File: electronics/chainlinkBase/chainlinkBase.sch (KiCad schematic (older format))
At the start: 50 parts, among them J101 Power In, J102 RELAY, J103 Power In, J104 RS485, J105 RS485, J106 Logic Power Out, J107 UART, J108 Output, J109 Output, J110 Output, J111 Conn_01x06_Male, J112 Conn_01x06_Male, SW101 SW_DIP_x04, U101 AP7361C-33E, U102 TPL7407L, U103 Buck, U104 TTGO_TDisplay, U105 MCP23017_SS, U106 SN74LV1T34DBV, U107 SP485, U108 SN74LV1T34DBV

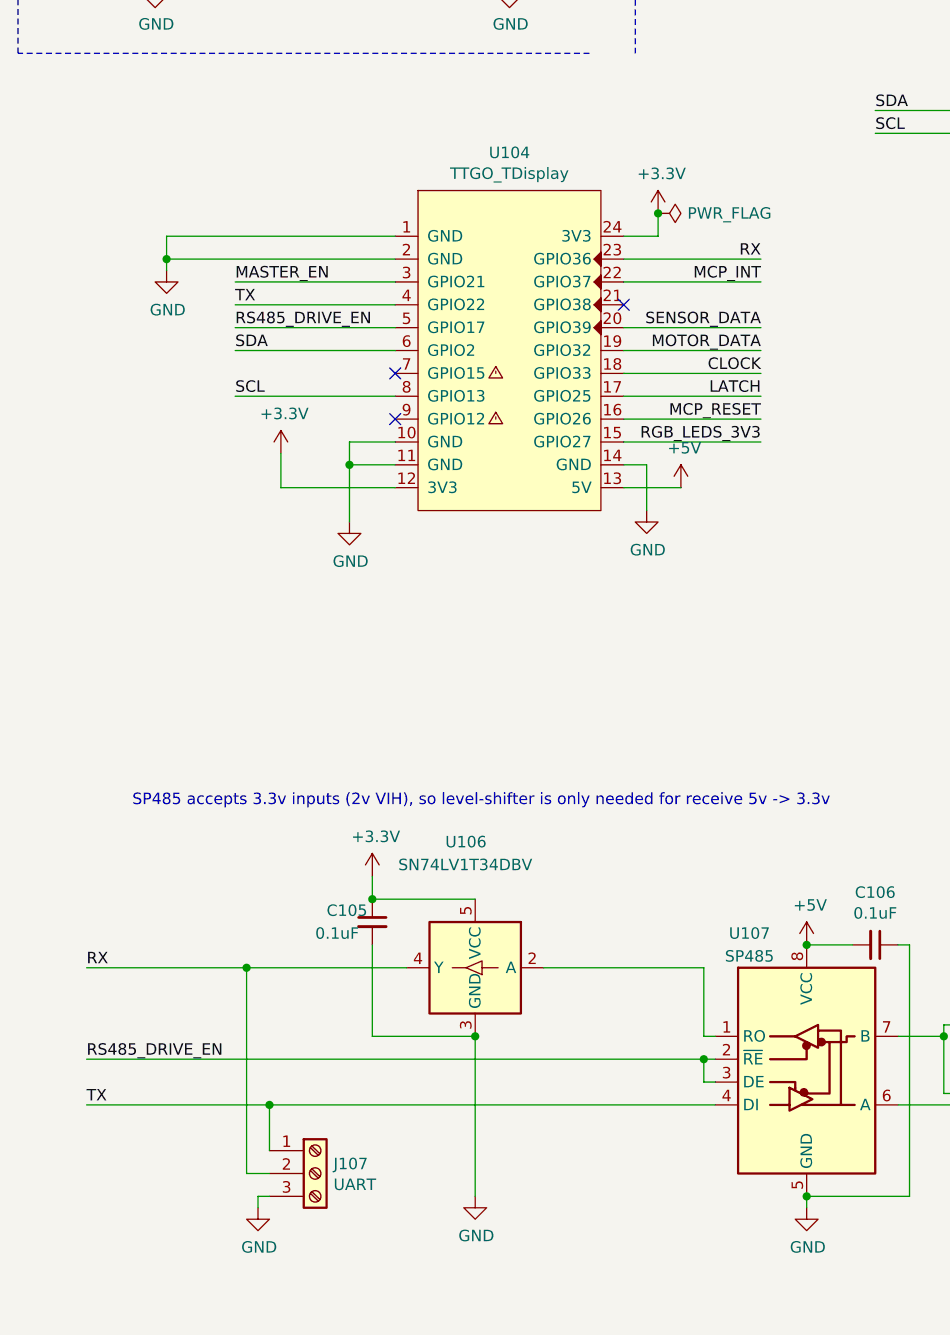
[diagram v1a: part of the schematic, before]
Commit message: More routing, CI
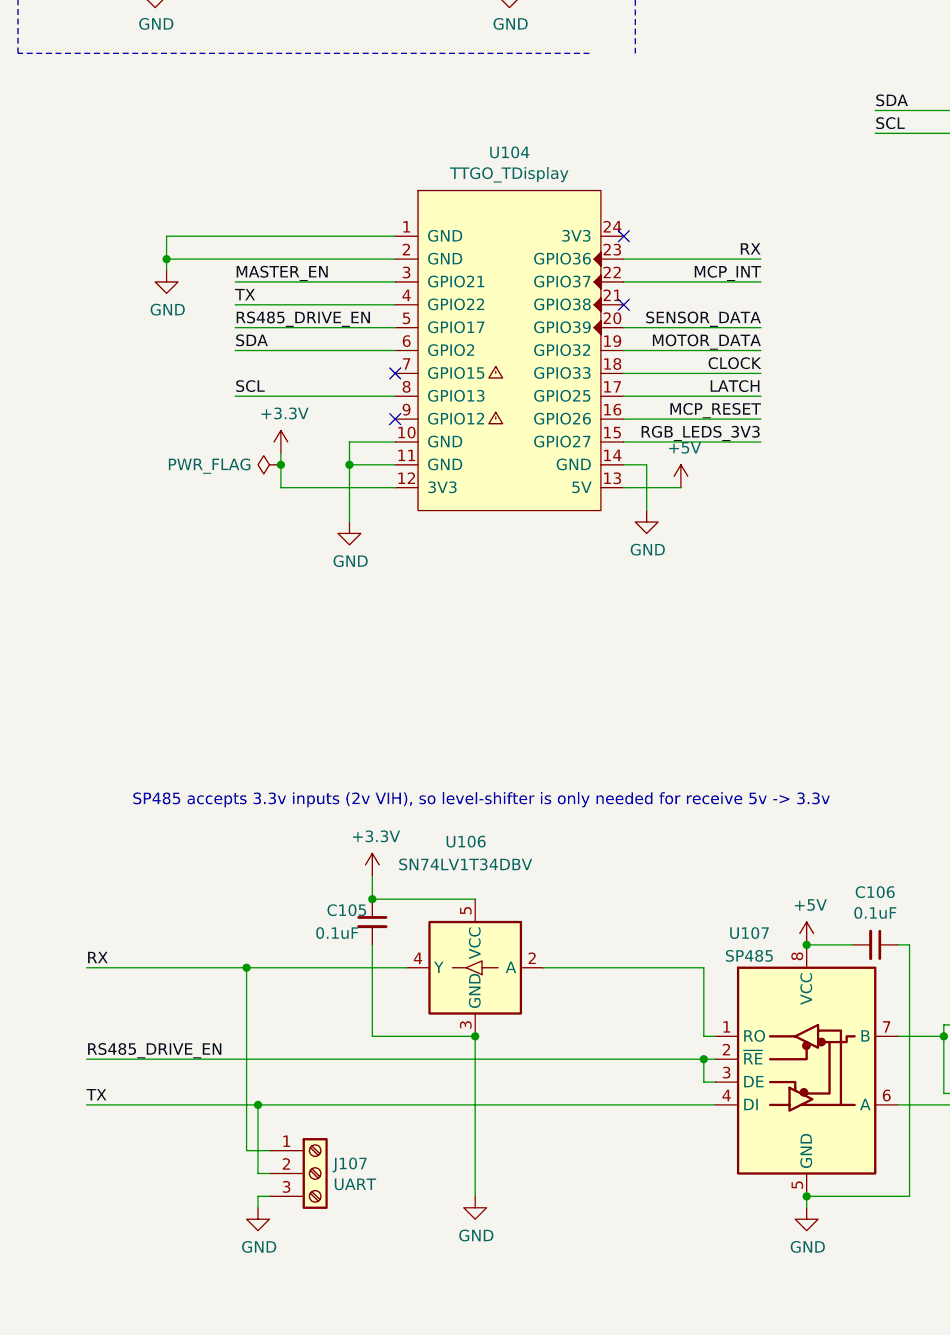
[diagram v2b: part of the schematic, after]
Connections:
- net +3V3: no longer U104.24 (3V3)
- net RX: now also J107.1 (Pin_1); no longer J107.2 (Pin_2)
- net TX: now also J107.2 (Pin_2); no longer J107.1 (Pin_1)
- no-connect marks 10 -> 11
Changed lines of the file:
@@
 	3350 4350 3950 4350
 Wire Wire Line
-	3500 3550 3500 3650
-Wire Wire Line
-	3500 3650 3350 3650
-Wire Wire Line
-	1850 4600 1850 4750
+	1850 4600 1850 4650
 Wire Wire Line
 	1850 4750 2350 4750
@@
 	1650 4050 2350 4050
 NoConn ~ 3350 3950
-$Comp
-L power:+3.3V #PWR0117
-U 1 1 60BD2B8F
-P 3500 3550
-F 0 "#PWR0117" H 3500 3400 50  0001 C CNN
-F 1 "+3.3V" H 3515 3723 50  0000 C CNN
-F 2 "" H 3500 3550 50  0001 C CNN
-F 3 "" H 3500 3550 50  0001 C CNN
-	1    3500 3550
-	1    0    0    -1
-$EndComp
 $Comp
 L power:+3.3V #PWR0122
@@
 Text Label 10350 1550 2    50   ~ 0
 RELAY_MASTER
-Wire Wire Line
-	1800 7450 1800 7650
-Connection ~ 1800 7450
-Wire Wire Line
-	1800 7450 3750 7450
-Wire Wire Line
-	1700 7750 1800 7750
 Wire Wire Line
 	1000 7250 3700 7250
@@
 Connection ~ 2250 6550
 Wire Wire Line
-	1000 7450 1800 7450
-Wire Wire Line
 	1000 6850 1700 6850
-Wire Wire Line
-	1700 7750 1700 6850
 Connection ~ 1700 6850
 Wire Wire Line
@@
 L power:PWR_FLAG #FLG0104
 U 1 1 61FD0285
-P 3500 3550
-F 0 "#FLG0104" H 3500 3625 50  0001 C CNN
-F 1 "PWR_FLAG" V 3500 3678 50  0000 L CNN
-F 2 "" H 3500 3550 50  0001 C CNN
-F 3 "~" H 3500 3550 50  0001 C CNN
-	1    3500 3550
-	0    1    1    0
-$EndComp
-Connection ~ 3500 3550
+P 1850 4650
+F 0 "#FLG0104" H 1850 4725 50  0001 C CNN
+F 1 "PWR_FLAG" V 1850 4778 50  0000 L CNN
+F 2 "" H 1850 4650 50  0001 C CNN
+F 3 "~" H 1850 4650 50  0001 C CNN
+	1    1850 4650
+	0    -1   -1   0
+$EndComp
 Text Label 10850 1550 0    50   ~ 0
 RELAY_MASTER
@@
 Wire Wire Line
 	8050 3000 8050 2950
+Connection ~ 1850 4650
+Wire Wire Line
+	1850 4650 1850 4750
+NoConn ~ 3350 3650
+Wire Wire Line
+	1000 7450 1750 7450
+Wire Wire Line
+	1700 7650 1800 7650
+Wire Wire Line
+	1700 7650 1700 6850
+Wire Wire Line
+	1750 7450 1750 7750
+Wire Wire Line
+	1750 7750 1800 7750
+Connection ~ 1750 7450
+Wire Wire Line
+	1750 7450 3750 7450
 $EndSCHEMATC
